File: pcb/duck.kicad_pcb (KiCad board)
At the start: 2 copper layers, 126.9 x 99.3 mm, 42 parts

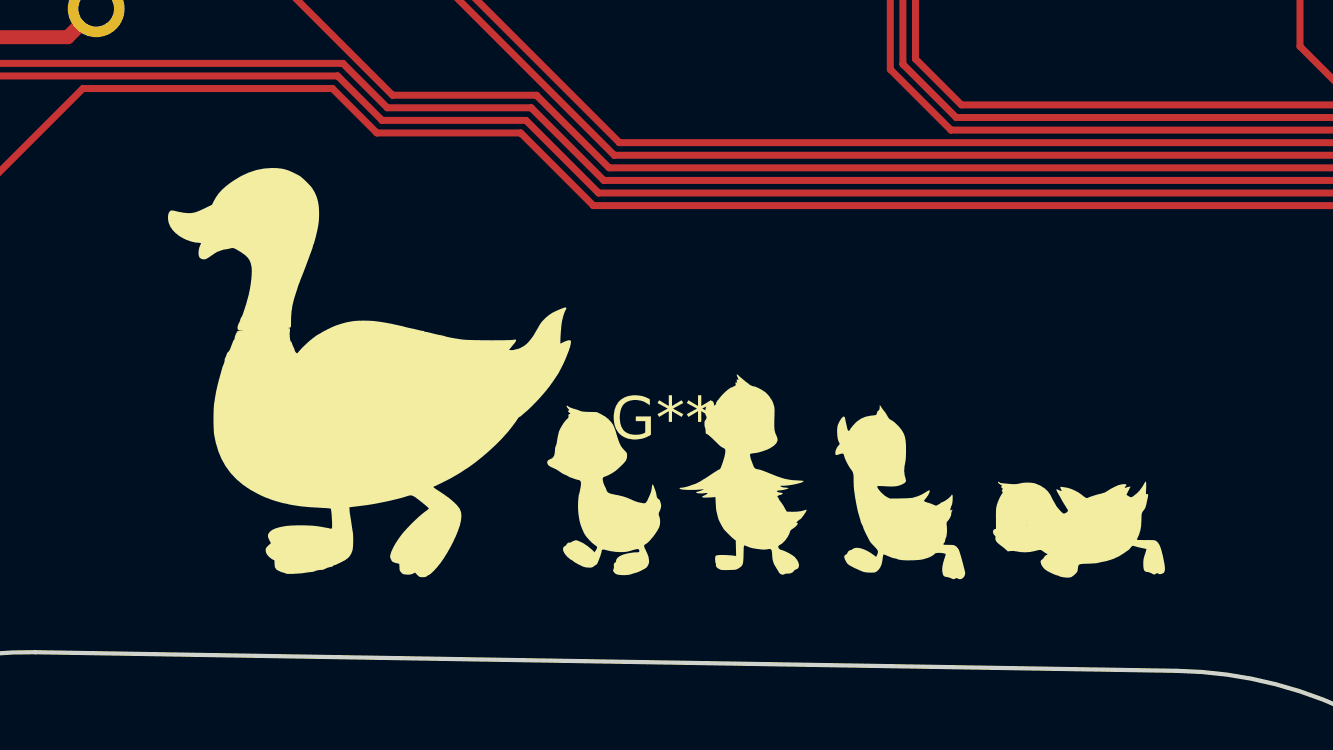
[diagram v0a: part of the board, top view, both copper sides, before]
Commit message: Duck is here
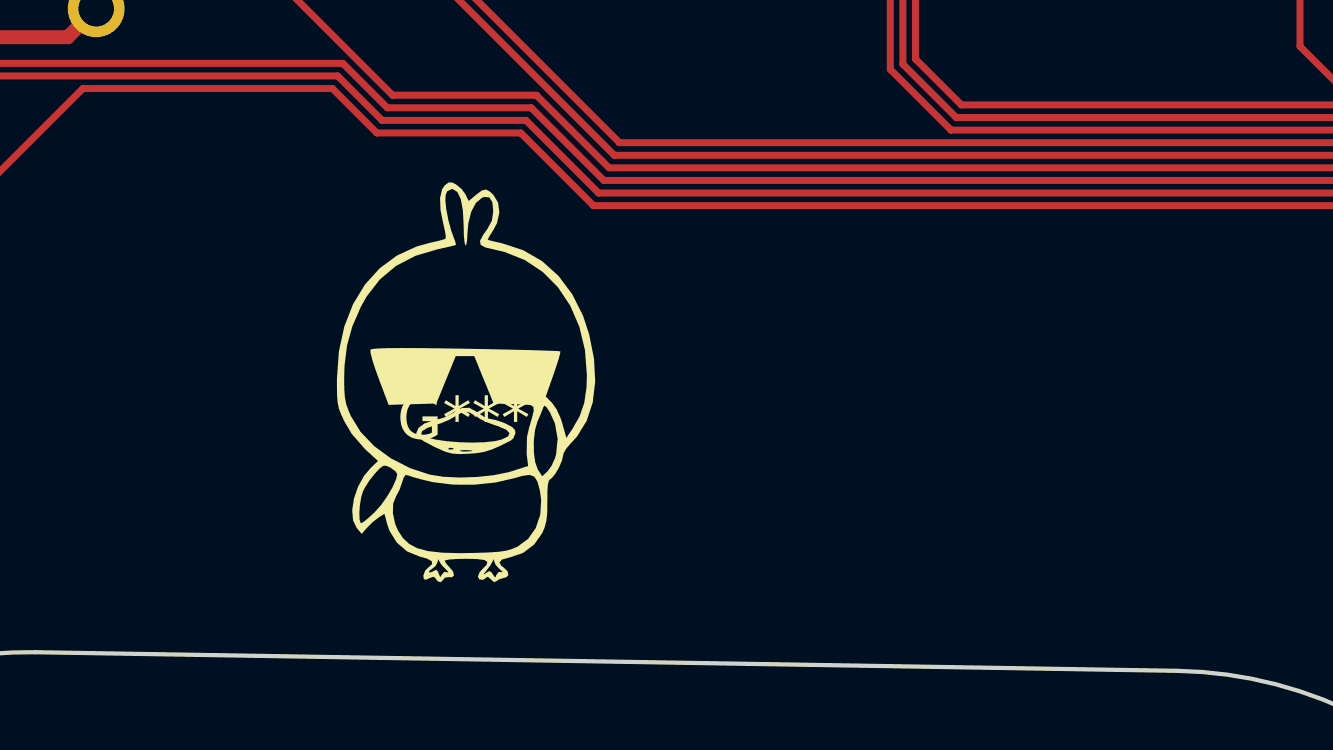
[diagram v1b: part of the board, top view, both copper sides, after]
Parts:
- removed the G*** at (99.1, -50.8) (x2)
- added G***: LOGO, LOGO, F.Cu at (91.4, -50.8)
- added G***: LOGO, LOGO, B.Cu at (91.4, -50.8)
